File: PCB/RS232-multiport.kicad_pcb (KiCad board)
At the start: 2 copper layers, 63.5 x 152.4 mm, 17 parts, among them J1 DB9_Male_MountingHoles, J2 DB9_Male_MountingHoles, J3 DB9_Male_MountingHoles, J4 DB9_Male_MountingHoles, U1 MAX232, U2 MAX232

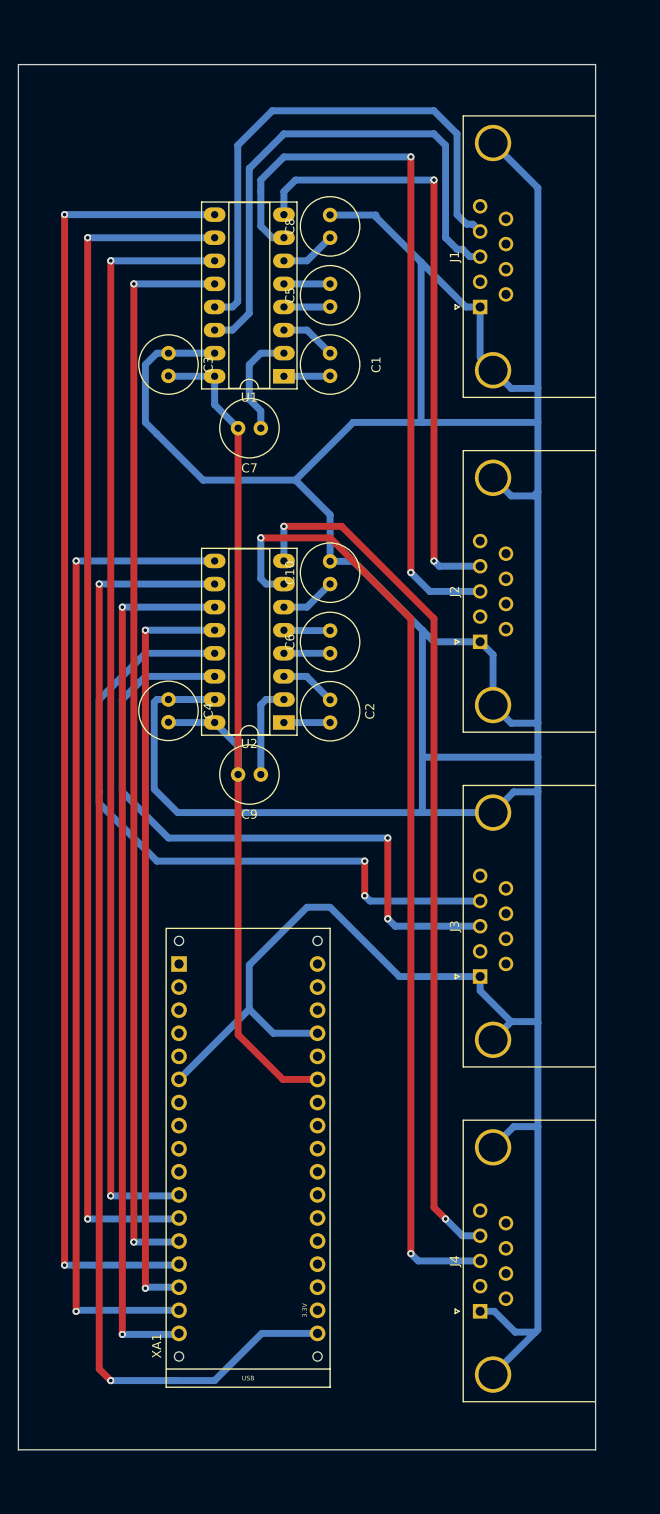
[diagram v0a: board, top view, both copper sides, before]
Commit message: v2
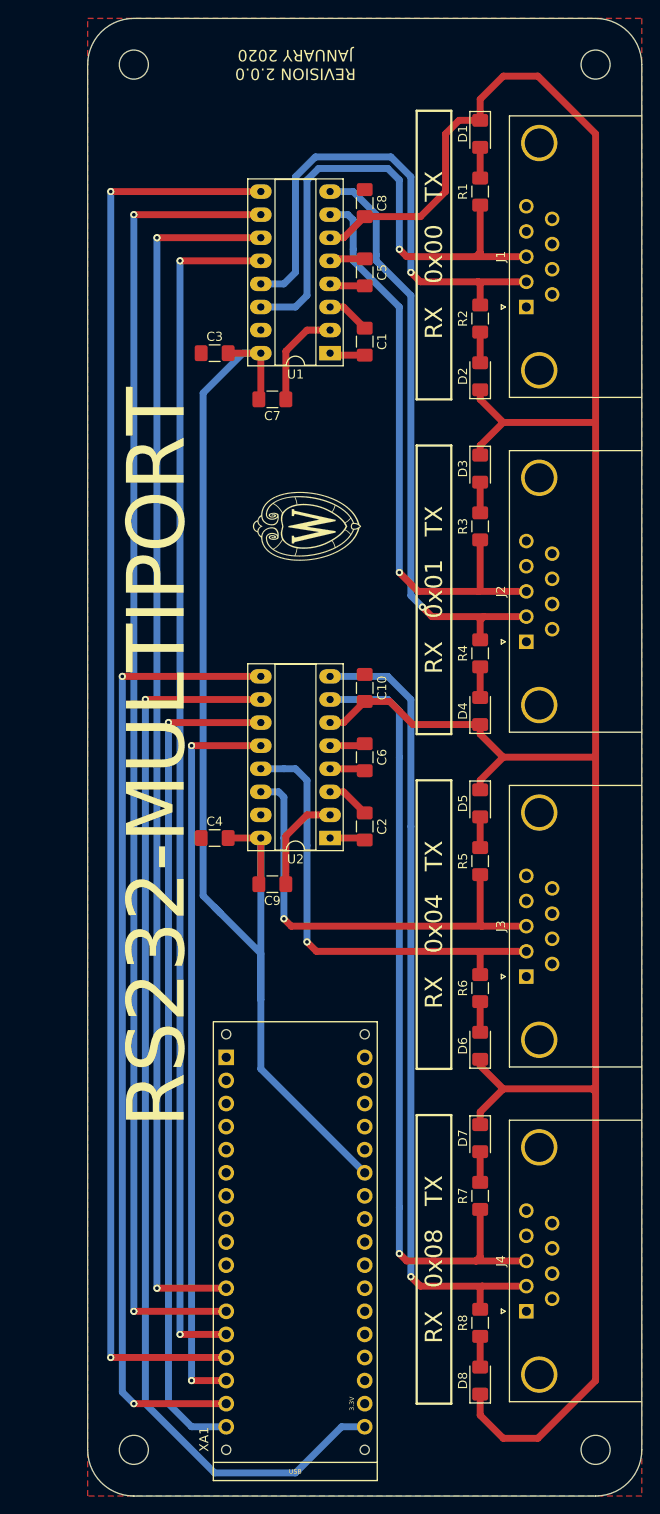
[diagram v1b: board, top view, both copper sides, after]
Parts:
- added D1: LED, LED_SMD:LED_1206_3216Metric_Pad1.42x1.75mm_HandSolder, F.Cu at (114.3, 33.0)
- added D2: LED, LED_SMD:LED_1206_3216Metric_Pad1.42x1.75mm_HandSolder, F.Cu at (114.3, 59.7)
- added D3: LED, LED_SMD:LED_1206_3216Metric_Pad1.42x1.75mm_HandSolder, F.Cu at (114.3, 69.8)
- added D4: LED, LED_SMD:LED_1206_3216Metric_Pad1.42x1.75mm_HandSolder, F.Cu at (114.3, 96.5)
- added D5: LED, LED_SMD:LED_1206_3216Metric_Pad1.42x1.75mm_HandSolder, F.Cu at (114.3, 106.7)
- added D6: LED, LED_SMD:LED_1206_3216Metric_Pad1.42x1.75mm_HandSolder, F.Cu at (114.3, 133.3)
- added D7: LED, LED_SMD:LED_1206_3216Metric_Pad1.42x1.75mm_HandSolder, F.Cu at (114.3, 143.5)
- added D8: LED, LED_SMD:LED_1206_3216Metric_Pad1.42x1.75mm_HandSolder, F.Cu at (114.3, 170.2)
- added G***: LOGO, footprints:logo, F.Cu at (95.2, 76.2)
- added R1: 4.7k, Resistor_SMD:R_1206_3216Metric_Pad1.42x1.75mm_HandSolder, F.Cu at (114.3, 39.4)
- added R2: 4.7k, Resistor_SMD:R_1206_3216Metric_Pad1.42x1.75mm_HandSolder, F.Cu at (114.3, 53.3)
- added R3: 4.7k, Resistor_SMD:R_1206_3216Metric_Pad1.42x1.75mm_HandSolder, F.Cu at (114.3, 76.2)
- added R4: 4.7k, Resistor_SMD:R_1206_3216Metric_Pad1.42x1.75mm_HandSolder, F.Cu at (114.3, 90.2)
- added R5: 4.7k, Resistor_SMD:R_1206_3216Metric_Pad1.42x1.75mm_HandSolder, F.Cu at (114.3, 113.0)
- added R6: 4.7k, Resistor_SMD:R_1206_3216Metric_Pad1.42x1.75mm_HandSolder, F.Cu at (114.3, 127.0)
- added R7: 4.7k, Resistor_SMD:R_1206_3216Metric_Pad1.42x1.75mm_HandSolder, F.Cu at (114.3, 149.9)
- added R8: 4.7k, Resistor_SMD:R_1206_3216Metric_Pad1.42x1.75mm_HandSolder, F.Cu at (114.3, 163.8)
- added REF**: MountingHole_3.2mm_M3, MountingHole:MountingHole_3.2mm_M3, F.Cu at (76.2, 25.4)
- added REF**: MountingHole_3.2mm_M3, MountingHole:MountingHole_3.2mm_M3, F.Cu at (76.2, 177.8)
- added REF**: MountingHole_3.2mm_M3, MountingHole:MountingHole_3.2mm_M3, F.Cu at (127.0, 177.8)
- added REF**: MountingHole_3.2mm_M3, MountingHole:MountingHole_3.2mm_M3, F.Cu at (127.0, 25.4)
- C1, C10, C2, C3, C4, C5, C6, C7, C8, C9: footprint Capacitor_THT:C_Radial_D6.3mm_H7.0mm_P2.50mm -> Capacitor_SMD:C_1206_3216Metric_Pad1.42x1.75mm_HandSolder
- moved C4 16.1 mm to (85.1, 110.5), turned to 0 degrees
- moved C2 14.4 mm to (101.6, 109.2)
- moved U2 13.7 mm to (97.8, 110.5)
- moved C9 12.1 mm to (91.4, 115.6)
- moved C10 12.0 mm to (101.6, 94.0)
- moved C6 12.0 mm to (101.6, 101.6)
- moved XA1 11.5 mm to (103.0, 179.2)
- moved U1 5.68 mm to (97.8, 57.1)
- moved C8 5.39 mm to (101.6, 40.6)
- moved C5 5.36 mm to (101.6, 48.3)
- moved C3 5.08 mm to (85.1, 57.1), turned to 0 degrees
- moved J1 5.08 mm to (119.4, 52.1)
- moved J2 5.08 mm to (119.4, 88.9)
- moved J3 5.08 mm to (119.4, 125.7)
- moved J4 5.08 mm to (119.4, 162.6)
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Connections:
- C10 pad 1: Net-(C10-Pad1) -> -10V
- C8 pad 1: Net-(C8-Pad1) -> -10V
- J1 pad 2: (no net) -> Net-(J1-Pad2)
- J1 pad 4: Net-(J1-Pad4) -> (no net)
- J2 pad 2: (no net) -> Net-(J2-Pad2)
- J2 pad 4: Net-(J2-Pad4) -> (no net)
- J3 pad 2: (no net) -> Net-(J3-Pad2)
- J3 pad 4: Net-(J3-Pad4) -> (no net)
- J4 pad 2: (no net) -> Net-(J4-Pad2)
- J4 pad 4: Net-(J4-Pad4) -> (no net)
- U1 pad 13: Net-(J1-Pad4) -> Net-(J1-Pad2)
- U1 pad 6: Net-(C8-Pad1) -> -10V
- U1 pad 8: Net-(J2-Pad4) -> Net-(J2-Pad2)
- U2 pad 13: Net-(J3-Pad4) -> Net-(J3-Pad2)
- U2 pad 6: Net-(C10-Pad1) -> -10V
- U2 pad 8: Net-(J4-Pad4) -> Net-(J4-Pad2)
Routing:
- net GND: track 478.5 -> 0.00 mm
- net -10V: track 0.00 -> 277.2 mm
- net Net-(J4-Pad4): track 95.7 -> 0.00 mm, vias 2 -> 0
- net Net-(J4-Pad2): track 0.00 -> 89.2 mm, vias 0 -> 1
- net Net-(J3-Pad4): track 74.8 -> 0.00 mm, vias 2 -> 0
- net Net-(J2-Pad4): track 66.8 -> 0.00 mm, vias 2 -> 0
- net Net-(J2-Pad2): track 0.00 -> 66.0 mm, vias 0 -> 1
- net Net-(J1-Pad4): track 58.9 -> 0.00 mm
- net Net-(J1-Pad2): track 0.00 -> 55.6 mm, vias 0 -> 1
- net Net-(J3-Pad2): track 0.00 -> 50.5 mm, vias 0 -> 1
- net +5V: track 101.3 -> 137.5 mm
- net Net-(J3-Pad3): track 72.1 -> 48.9 mm, vias 2 -> 1
- net Net-(J4-Pad3): track 105.3 -> 88.0 mm, vias 2 -> 1
- net Net-(J2-Pad3): track 79.9 -> 64.3 mm, vias 2 -> 1
- net Net-(U1-Pad12): track 119.3 -> 132.1 mm
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- added copper zone on F.Cu, net GND
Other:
- board size 63.5 x 152.4 mm -> 61 x 162.6 mm
- board text added: "BLAISE THOMPSON UW-MADISON DEPARTMENT OF CHEMISTRY"
- board text added: "REVISION 2.0.0 JANUARY 2020"
- board text added: "RS232-MULTIPORT"
- board text added: "RX 0x00 TX"
- board text added: "RX 0x01 TX"
- board text added: "RX 0x04 TX"
- board text added: "RX 0x08 TX"
